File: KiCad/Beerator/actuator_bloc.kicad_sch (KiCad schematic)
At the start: 26 parts, among them U501 Servo

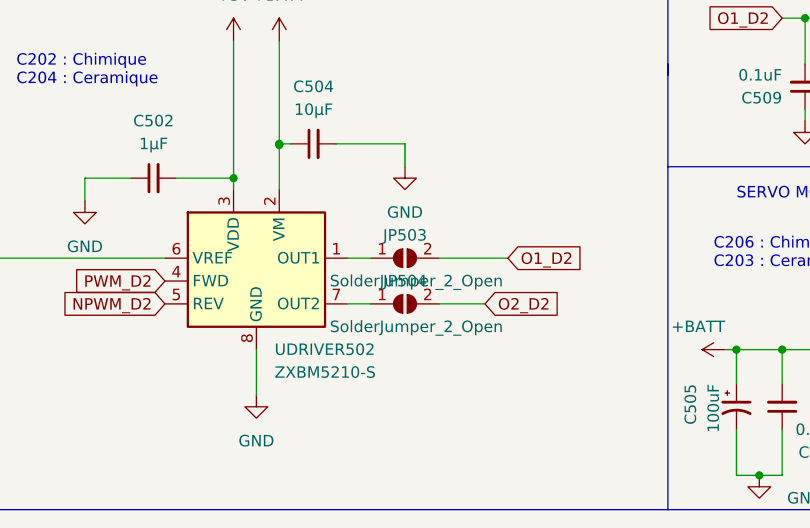
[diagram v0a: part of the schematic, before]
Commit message: pcb_v2
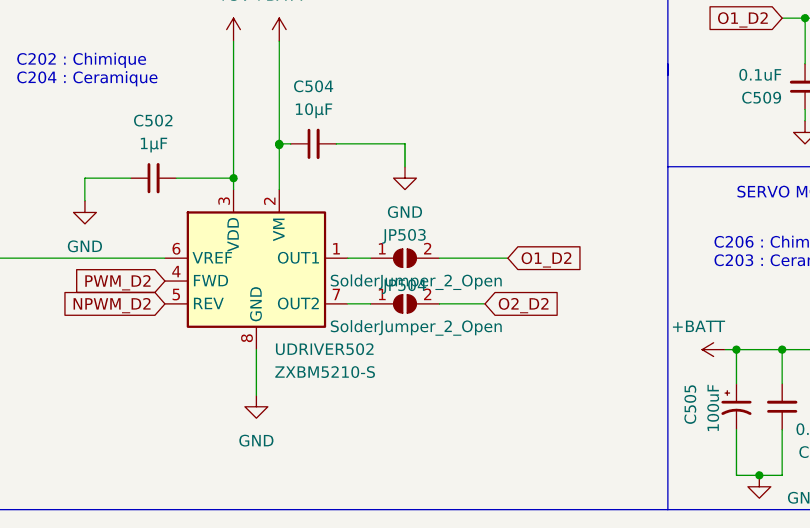
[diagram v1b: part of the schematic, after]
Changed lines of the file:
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@@
   (symbol (lib_id "Jumper:SolderJumper_2_Open") (at 96.52 128.27 0) (unit 1)
     (in_bom yes) (on_board yes)
-    (property "Reference" "JP504" (id 0) (at 96.52 125.73 0))
+    (property "Reference" "JP504" (id 0) (at 96.52 126.238 0))
     (property "Value" "SolderJumper_2_Open" (id 1) (at 97.79 130.81 0))
     (property "Footprint" "Jumper:SolderJumper-3_P2.0mm_Open_TrianglePad1.0x1.5mm" (id 2) (at 96.52 128.27 0)
